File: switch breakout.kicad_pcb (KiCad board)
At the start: 2 copper layers, 2 parts

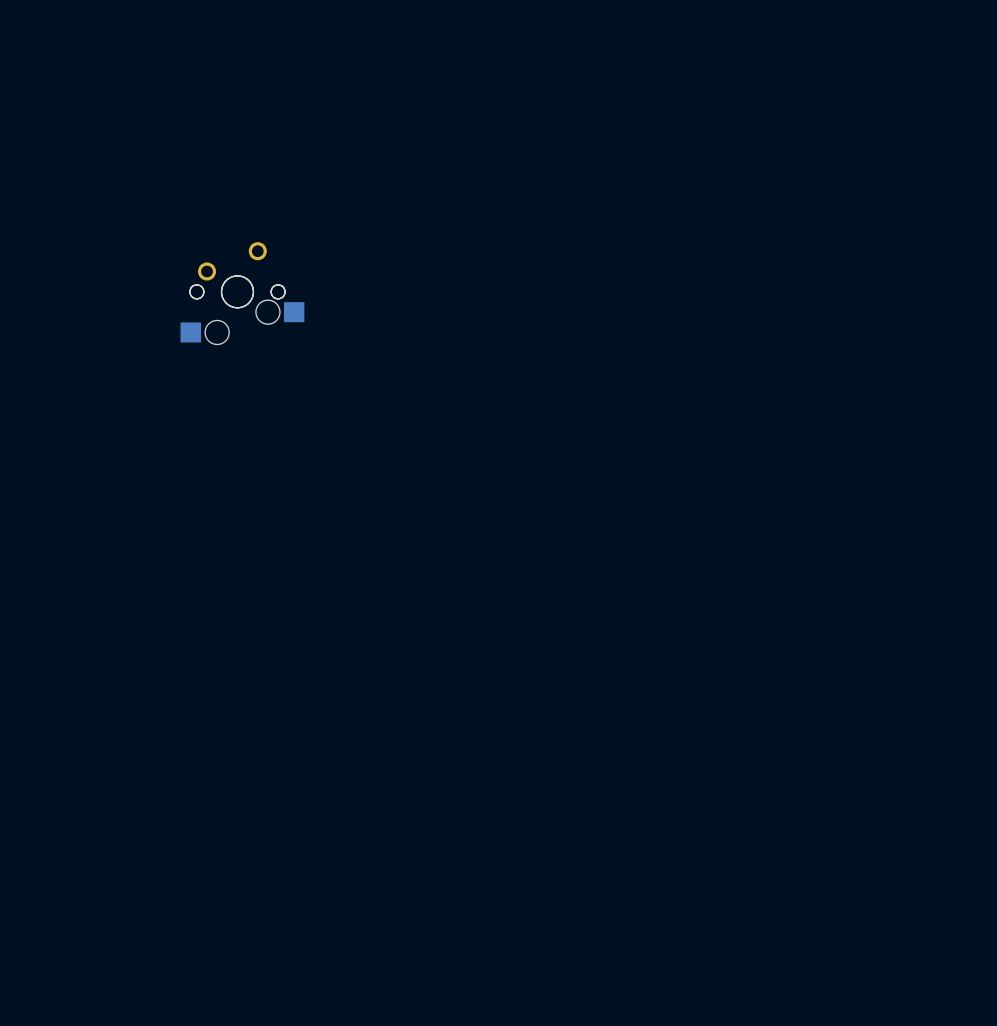
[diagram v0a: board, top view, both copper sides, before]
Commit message: update
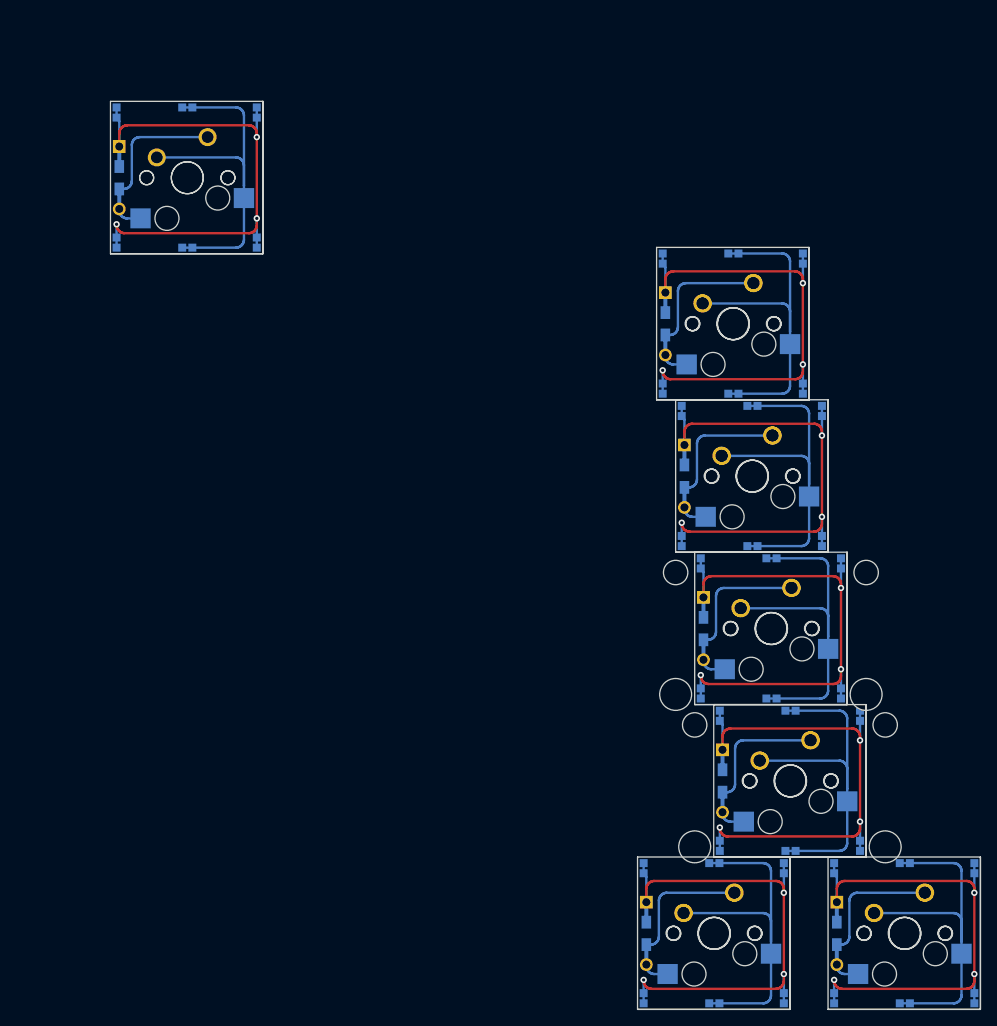
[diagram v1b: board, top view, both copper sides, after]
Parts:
- removed the MX1 at (41.3, 49.2)
- removed the REF** at (41.3, 49.2)
- added D1: 1N4148W, Keebio-Parts:Diode-dual - Copy, B.Cu at (116.2, 129.4)
- added D1: 1N4148W, Keebio-Parts:Diode-dual - Copy, B.Cu at (92.4, 129.4)
- added D1: 1N4148W, Keebio-Parts:Diode-dual - Copy, B.Cu at (101.9, 110.4)
- added D1: 1N4148W, Keebio-Parts:Diode-dual - Copy, B.Cu at (99.5, 91.3)
- added D1: 1N4148W, Keebio-Parts:Diode-dual - Copy, B.Cu at (97.1, 72.3)
- added D1: 1N4148W, Keebio-Parts:Diode-dual - Copy, B.Cu at (94.8, 53.2)
- added D1: 1N4148W, Keebio-Parts:Diode-dual - Copy, B.Cu at (26.5, 34.9)
- added MX1: MX-NoLED, MX_Only:MXOnly-1U-NoLED, F.Cu at (124.7, 129.4)
- added MX1: MX-NoLED, MX_Only:MXOnly-1U-NoLED, F.Cu at (100.9, 129.4)
- added MX1: MX-NoLED, MX_Only:MXOnly-1U-NoLED, F.Cu at (110.4, 110.4)
- added MX1: MX-NoLED, MX_Only:MXOnly-1U-NoLED, F.Cu at (108.0, 91.3)
- added MX1: MX-NoLED, MX_Only:MXOnly-1U-NoLED, F.Cu at (105.6, 72.3)
- added MX1: MX-NoLED, MX_Only:MXOnly-1U-NoLED, F.Cu at (103.3, 53.2)
- added MX1: MX-NoLED, MX_Only:MXOnly-1U-NoLED, F.Cu at (35.0, 34.9)
- added MX2: MX-NoLED, MX_Only:MXOnly-1U-Hotswap, F.Cu at (124.7, 129.4)
- added MX2: MX-NoLED, MX_Only:MXOnly-1U-Hotswap, F.Cu at (100.9, 129.4)
- added MX2: MX-NoLED, MX_Only:MXOnly-1U-Hotswap, F.Cu at (110.4, 110.4)
- added MX2: MX-NoLED, MX_Only:MXOnly-1U-Hotswap, F.Cu at (108.0, 91.3)
- added MX2: MX-NoLED, MX_Only:MXOnly-1U-Hotswap, F.Cu at (105.6, 72.3)
- added MX2: MX-NoLED, MX_Only:MXOnly-1U-Hotswap, F.Cu at (103.3, 53.2)
- added MX2: MX-NoLED, MX_Only:MXOnly-1U-Hotswap, F.Cu at (35.0, 34.9)
- added REF**: Jumper-UserFriendly, random-keyboard-parts:Jumper-UserFriendly, B.Cu at (115.9, 121.4)
- added REF**: Jumper-UserFriendly, random-keyboard-parts:Jumper-UserFriendly, B.Cu at (92.0, 121.4)
- added REF**: Jumper-UserFriendly, random-keyboard-parts:Jumper-UserFriendly, B.Cu at (109.6, 137.6)
- added REF**: Jumper-UserFriendly, random-keyboard-parts:Jumper-UserFriendly, B.Cu at (109.6, 121.4)
- added REF**: Jumper-UserFriendly, random-keyboard-parts:Jumper-UserFriendly, B.Cu at (101.6, 118.6)
- added REF**: Jumper-UserFriendly, random-keyboard-parts:Jumper-UserFriendly, B.Cu at (119.1, 118.6)
- added REF**: Jumper-UserFriendly, random-keyboard-parts:Jumper-UserFriendly, B.Cu at (110.5, 119.1)
- added REF**: Jumper-UserFriendly, random-keyboard-parts:Jumper-UserFriendly, B.Cu at (110.5, 101.6)
- added REF**: Jumper-UserFriendly, random-keyboard-parts:Jumper-UserFriendly, B.Cu at (119.1, 102.3)
- added REF**: Jumper-UserFriendly, random-keyboard-parts:Jumper-UserFriendly, B.Cu at (101.6, 102.3)
- added REF**: Jumper-UserFriendly, random-keyboard-parts:Jumper-UserFriendly, B.Cu at (99.2, 99.5)
- added REF**: Jumper-UserFriendly, random-keyboard-parts:Jumper-UserFriendly, B.Cu at (133.4, 121.4)
- added REF**: Jumper-UserFriendly, random-keyboard-parts:Jumper-UserFriendly, B.Cu at (99.2, 83.3)
- added REF**: Jumper-UserFriendly, random-keyboard-parts:Jumper-UserFriendly, B.Cu at (116.7, 99.5)
- added REF**: Jumper-UserFriendly, random-keyboard-parts:Jumper-UserFriendly, B.Cu at (116.7, 83.3)
- added REF**: Jumper-UserFriendly, random-keyboard-parts:Jumper-UserFriendly, B.Cu at (108.2, 100.0)
- added REF**: Jumper-UserFriendly, random-keyboard-parts:Jumper-UserFriendly, B.Cu at (108.2, 82.5)
- added REF**: Jumper-UserFriendly, random-keyboard-parts:Jumper-UserFriendly, B.Cu at (96.8, 80.5)
- added REF**: Jumper-UserFriendly, random-keyboard-parts:Jumper-UserFriendly, B.Cu at (96.8, 64.2)
- added REF**: Jumper-UserFriendly, random-keyboard-parts:Jumper-UserFriendly, B.Cu at (114.3, 80.5)
- added REF**: Jumper-UserFriendly, random-keyboard-parts:Jumper-UserFriendly, B.Cu at (114.3, 64.2)
- added REF**: Jumper-UserFriendly, random-keyboard-parts:Jumper-UserFriendly, B.Cu at (105.8, 63.5)
- added REF**: Jumper-UserFriendly, random-keyboard-parts:Jumper-UserFriendly, B.Cu at (133.4, 137.6)
- added REF**: Jumper-UserFriendly, random-keyboard-parts:Jumper-UserFriendly, B.Cu at (105.8, 81.0)
- added REF**: Jumper-UserFriendly, random-keyboard-parts:Jumper-UserFriendly, B.Cu at (94.4, 61.4)
- added REF**: Jumper-UserFriendly, random-keyboard-parts:Jumper-UserFriendly, B.Cu at (94.4, 45.2)
- added REF**: Jumper-UserFriendly, random-keyboard-parts:Jumper-UserFriendly, B.Cu at (112.0, 61.4)
- added REF**: Jumper-UserFriendly, random-keyboard-parts:Jumper-UserFriendly, B.Cu at (112.0, 45.2)
- added REF**: Jumper-UserFriendly, random-keyboard-parts:Jumper-UserFriendly, B.Cu at (103.4, 61.9)
- added REF**: Jumper-UserFriendly, random-keyboard-parts:Jumper-UserFriendly, B.Cu at (103.4, 44.4)
- added REF**: 2U, MX_Only:MXOnly-2U-NoLED, F.Cu at (108.0, 91.3)
- added REF**: 1.25U, MX_Only:MXOnly-1.25U-NoLED, F.Cu at (124.6, 129.4)
- added REF**: 1.25U, MX_Only:MXOnly-1.25U-NoLED, F.Cu at (100.8, 129.4)
- added REF**: Jumper-UserFriendly, random-keyboard-parts:Jumper-UserFriendly, B.Cu at (124.8, 120.6)
- added REF**: 2.25U, MX_Only:MXOnly-2.25U-NoLED, F.Cu at (110.3, 110.3)
- added REF**: 1.75U, MX_Only:MXOnly-1.75U-NoLED, F.Cu at (105.6, 72.2)
- added REF**: 1.5U, MX_Only:MXOnly-1.5U-NoLED, F.Cu at (103.2, 53.2)
- added REF**: Jumper-UserFriendly, random-keyboard-parts:Jumper-UserFriendly, B.Cu at (35.1, 26.2)
- added REF**: Jumper-UserFriendly, random-keyboard-parts:Jumper-UserFriendly, B.Cu at (35.1, 43.7)
- added REF**: Jumper-UserFriendly, random-keyboard-parts:Jumper-UserFriendly, B.Cu at (26.2, 43.2)
- added REF**: Jumper-UserFriendly, random-keyboard-parts:Jumper-UserFriendly, B.Cu at (26.2, 26.9)
- added REF**: Jumper-UserFriendly, random-keyboard-parts:Jumper-UserFriendly, B.Cu at (43.7, 26.9)
- added REF**: Jumper-UserFriendly, random-keyboard-parts:Jumper-UserFriendly, B.Cu at (43.7, 43.2)
- added REF**: Jumper-UserFriendly, random-keyboard-parts:Jumper-UserFriendly, B.Cu at (115.9, 137.6)
- added REF**: Jumper-UserFriendly, random-keyboard-parts:Jumper-UserFriendly, B.Cu at (124.8, 138.1)
- added REF**: Jumper-UserFriendly, random-keyboard-parts:Jumper-UserFriendly, B.Cu at (92.0, 137.6)
- added REF**: Jumper-UserFriendly, random-keyboard-parts:Jumper-UserFriendly, B.Cu at (101.0, 120.6)
- added REF**: Jumper-UserFriendly, random-keyboard-parts:Jumper-UserFriendly, B.Cu at (101.0, 138.1)
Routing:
- net Net-(D1-Pad1): track 0.00 -> 458.9 mm, vias 0 -> 21
- net Net-(MX1-Pad1): track 0.00 -> 322.7 mm
- net Net-(D1-Pad2): track 0.00 -> 140.5 mm
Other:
- board outline added: 108.7 x 113.5 mm
- board text added: "COL"
- board text added: "ROW"

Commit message: update
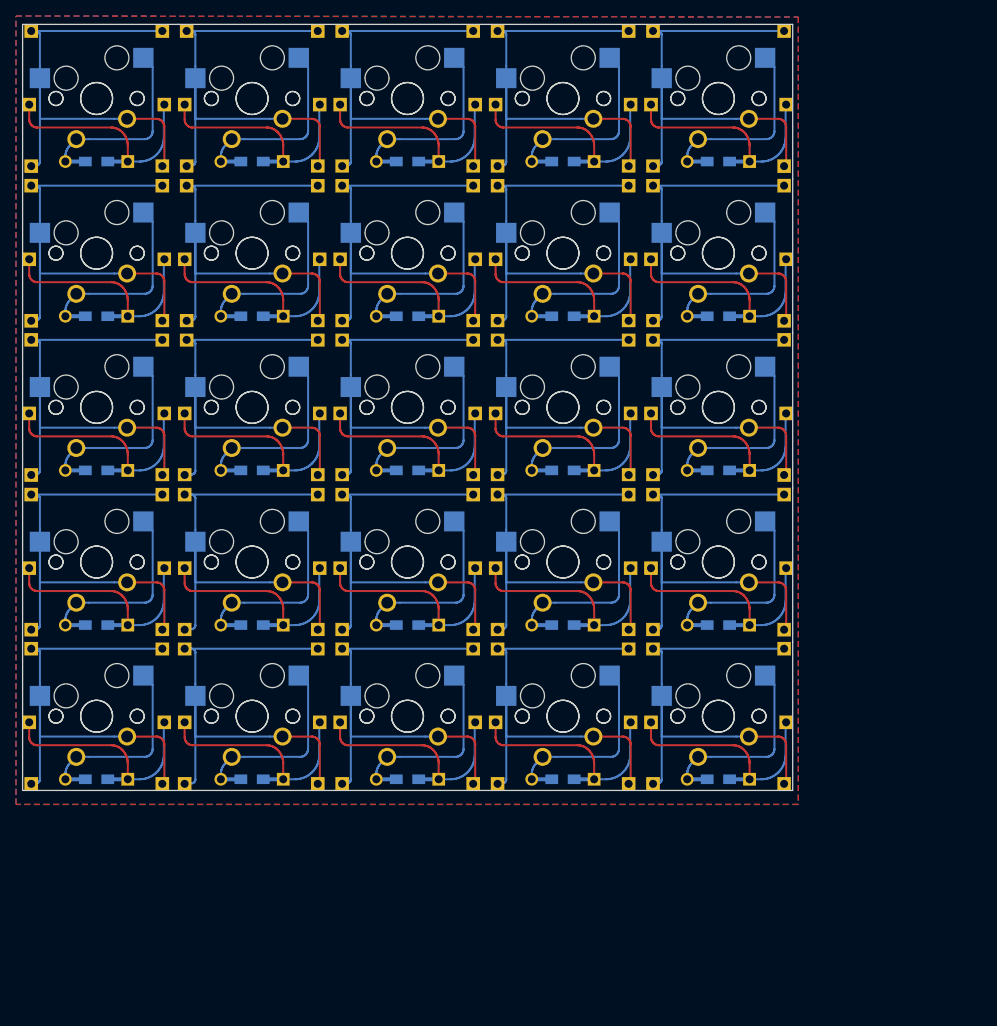
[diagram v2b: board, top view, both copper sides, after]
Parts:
- removed the D1 at (116.2, 129.4)
- removed the D1 at (92.4, 129.4)
- removed the D1 at (101.9, 110.4)
- removed the D1 at (99.5, 91.3)
- removed the D1 at (97.1, 72.3)
- removed the D1 at (94.8, 53.2)
- removed the D1 at (26.5, 34.9)
- removed the MX1 at (124.7, 129.4)
- removed the MX1 at (100.9, 129.4)
- removed the MX1 at (110.4, 110.4)
- removed the MX1 at (108.0, 91.3)
- removed the MX1 at (105.6, 72.3)
- removed the MX1 at (103.3, 53.2)
- removed the MX1 at (35.0, 34.9)
- removed the MX2 at (124.7, 129.4)
- removed the MX2 at (100.9, 129.4)
- removed the MX2 at (110.4, 110.4)
- removed the MX2 at (108.0, 91.3)
- removed the MX2 at (105.6, 72.3)
- removed the MX2 at (103.3, 53.2)
- removed the MX2 at (35.0, 34.9)
- removed the REF** at (115.9, 121.4)
- removed the REF** at (92.0, 121.4)
- removed the REF** at (109.6, 137.6)
- removed the REF** at (109.6, 121.4)
- removed the REF** at (101.6, 118.6)
- removed the REF** at (119.1, 118.6)
- removed the REF** at (110.5, 119.1)
- removed the REF** at (110.5, 101.6)
- removed the REF** at (119.1, 102.3)
- removed the REF** at (101.6, 102.3)
- removed the REF** at (99.2, 99.5)
- removed the REF** at (133.4, 121.4)
- removed the REF** at (99.2, 83.3)
- removed the REF** at (116.7, 99.5)
- removed the REF** at (116.7, 83.3)
- removed the REF** at (108.2, 100.0)
- removed the REF** at (108.2, 82.5)
- removed the REF** at (96.8, 80.5)
- removed the REF** at (96.8, 64.2)
- removed the REF** at (114.3, 80.5)
- removed the REF** at (114.3, 64.2)
- removed the REF** at (105.8, 63.5)
- removed the REF** at (133.4, 137.6)
- removed the REF** at (105.8, 81.0)
- removed the REF** at (94.4, 61.4)
- removed the REF** at (94.4, 45.2)
- removed the REF** at (112.0, 61.4)
- removed the REF** at (112.0, 45.2)
- removed the REF** at (103.4, 61.9)
- removed the REF** at (103.4, 44.4)
- removed the REF** at (108.0, 91.3)
- removed the REF** at (124.6, 129.4)
- removed the REF** at (100.8, 129.4)
- removed the REF** at (124.8, 120.6)
- removed the REF** at (110.3, 110.3)
- removed the REF** at (105.6, 72.2)
- removed the REF** at (103.2, 53.2)
- removed the REF** at (35.1, 26.2)
- removed the REF** at (35.1, 43.7)
- removed the REF** at (26.2, 43.2)
- removed the REF** at (26.2, 26.9)
- removed the REF** at (43.7, 26.9)
- removed the REF** at (43.7, 43.2)
- removed the REF** at (115.9, 137.6)
- removed the REF** at (124.8, 138.1)
- removed the REF** at (92.0, 137.6)
- removed the REF** at (101.0, 120.6)
- removed the REF** at (101.0, 138.1)
- added D1: 1N4148W, Keebio-Parts:Diode-dual - Copy, B.Cu at (62.5, 110.1)
- added D1: 1N4148W, Keebio-Parts:Diode-dual - Copy, B.Cu at (43.1, 71.5)
- added D1: 1N4148W, Keebio-Parts:Diode-dual - Copy, B.Cu at (101.4, 90.9)
- added D1: 1N4148W, Keebio-Parts:Diode-dual - Copy, B.Cu at (101.4, 71.5)
- added D1: 1N4148W, Keebio-Parts:Diode-dual - Copy, B.Cu at (82.0, 90.9)
- added D1: 1N4148W, Keebio-Parts:Diode-dual - Copy, B.Cu at (82.0, 71.5)
- added D1: 1N4148W, Keebio-Parts:Diode-dual - Copy, B.Cu at (23.7, 71.5)
- added D1: 1N4148W, Keebio-Parts:Diode-dual - Copy, B.Cu at (101.4, 52.3)
- added D1: 1N4148W, Keebio-Parts:Diode-dual - Copy, B.Cu at (101.4, 32.9)
- added D1: 1N4148W, Keebio-Parts:Diode-dual - Copy, B.Cu at (82.0, 52.3)
- added D1: 1N4148W, Keebio-Parts:Diode-dual - Copy, B.Cu at (82.0, 32.9)
- added D1: 1N4148W, Keebio-Parts:Diode-dual - Copy, B.Cu at (43.1, 110.1)
- added D1: 1N4148W, Keebio-Parts:Diode-dual - Copy, B.Cu at (62.5, 52.3)
- added D1: 1N4148W, Keebio-Parts:Diode-dual - Copy, B.Cu at (62.5, 32.9)
- added D1: 1N4148W, Keebio-Parts:Diode-dual - Copy, B.Cu at (43.1, 52.3)
- added D1: 1N4148W, Keebio-Parts:Diode-dual - Copy, B.Cu at (23.7, 52.3)
- added D1: 1N4148W, Keebio-Parts:Diode-dual - Copy, B.Cu at (43.1, 32.9)
- added D1: 1N4148W, Keebio-Parts:Diode-dual - Copy, B.Cu at (23.7, 32.9)
- added D1: 1N4148W, Keebio-Parts:Diode-dual - Copy, B.Cu at (101.4, 110.1)
- added D1: 1N4148W, Keebio-Parts:Diode-dual - Copy, B.Cu at (23.7, 110.1)
- added D1: 1N4148W, Keebio-Parts:Diode-dual - Copy, B.Cu at (82.0, 110.1)
- added D1: 1N4148W, Keebio-Parts:Diode-dual - Copy, B.Cu at (62.5, 90.9)
- added D1: 1N4148W, Keebio-Parts:Diode-dual - Copy, B.Cu at (62.5, 71.5)
- added D1: 1N4148W, Keebio-Parts:Diode-dual - Copy, B.Cu at (23.7, 90.9)
- added D1: 1N4148W, Keebio-Parts:Diode-dual - Copy, B.Cu at (43.1, 90.9)
- added MX1: MX-NoLED, MX_Only:MXOnly-1U-NoLED, F.Cu at (62.5, 102.3)
- added MX1: MX-NoLED, MX_Only:MXOnly-1U-NoLED, F.Cu at (43.1, 63.7)
- added MX1: MX-NoLED, MX_Only:MXOnly-1U-NoLED, F.Cu at (101.4, 83.0)
- added MX1: MX-NoLED, MX_Only:MXOnly-1U-NoLED, F.Cu at (101.4, 63.7)
- added MX1: MX-NoLED, MX_Only:MXOnly-1U-NoLED, F.Cu at (82.0, 83.0)
- added MX1: MX-NoLED, MX_Only:MXOnly-1U-NoLED, F.Cu at (82.0, 63.7)
- added MX1: MX-NoLED, MX_Only:MXOnly-1U-NoLED, F.Cu at (23.7, 63.7)
- added MX1: MX-NoLED, MX_Only:MXOnly-1U-NoLED, F.Cu at (101.4, 44.4)
- added MX1: MX-NoLED, MX_Only:MXOnly-1U-NoLED, F.Cu at (101.4, 25.0)
- added MX1: MX-NoLED, MX_Only:MXOnly-1U-NoLED, F.Cu at (82.0, 25.0)
- added MX1: MX-NoLED, MX_Only:MXOnly-1U-NoLED, F.Cu at (82.0, 44.4)
- added MX1: MX-NoLED, MX_Only:MXOnly-1U-NoLED, F.Cu at (101.4, 102.3)
- added MX1: MX-NoLED, MX_Only:MXOnly-1U-NoLED, F.Cu at (62.5, 25.0)
- added MX1: MX-NoLED, MX_Only:MXOnly-1U-NoLED, F.Cu at (62.5, 44.4)
- added MX1: MX-NoLED, MX_Only:MXOnly-1U-NoLED, F.Cu at (43.1, 44.4)
- added MX1: MX-NoLED, MX_Only:MXOnly-1U-NoLED, F.Cu at (23.7, 44.4)
- added MX1: MX-NoLED, MX_Only:MXOnly-1U-NoLED, F.Cu at (43.1, 25.0)
- added MX1: MX-NoLED, MX_Only:MXOnly-1U-NoLED, F.Cu at (23.7, 25.0)
- added MX1: MX-NoLED, MX_Only:MXOnly-1U-NoLED, F.Cu at (43.1, 102.3)
- added MX1: MX-NoLED, MX_Only:MXOnly-1U-NoLED, F.Cu at (82.0, 102.3)
- added MX1: MX-NoLED, MX_Only:MXOnly-1U-NoLED, F.Cu at (23.7, 102.3)
- added MX1: MX-NoLED, MX_Only:MXOnly-1U-NoLED, F.Cu at (62.5, 63.7)
- added MX1: MX-NoLED, MX_Only:MXOnly-1U-NoLED, F.Cu at (62.5, 83.0)
- added MX1: MX-NoLED, MX_Only:MXOnly-1U-NoLED, F.Cu at (43.1, 83.0)
- added MX1: MX-NoLED, MX_Only:MXOnly-1U-NoLED, F.Cu at (23.7, 83.0)
- added MX2: MX-NoLED, MX_Only:MXOnly-1U-Hotswap, F.Cu at (82.0, 25.0)
- added MX2: MX-NoLED, MX_Only:MXOnly-1U-Hotswap, F.Cu at (43.1, 83.0)
- added MX2: MX-NoLED, MX_Only:MXOnly-1U-Hotswap, F.Cu at (43.1, 63.7)
- added MX2: MX-NoLED, MX_Only:MXOnly-1U-Hotswap, F.Cu at (101.4, 63.7)
- added MX2: MX-NoLED, MX_Only:MXOnly-1U-Hotswap, F.Cu at (101.4, 83.0)
- added MX2: MX-NoLED, MX_Only:MXOnly-1U-Hotswap, F.Cu at (82.0, 83.0)
- added MX2: MX-NoLED, MX_Only:MXOnly-1U-Hotswap, F.Cu at (82.0, 63.7)
- added MX2: MX-NoLED, MX_Only:MXOnly-1U-Hotswap, F.Cu at (23.7, 63.7)
- added MX2: MX-NoLED, MX_Only:MXOnly-1U-Hotswap, F.Cu at (101.4, 44.4)
- added MX2: MX-NoLED, MX_Only:MXOnly-1U-Hotswap, F.Cu at (101.4, 25.0)
- added MX2: MX-NoLED, MX_Only:MXOnly-1U-Hotswap, F.Cu at (82.0, 44.4)
- added MX2: MX-NoLED, MX_Only:MXOnly-1U-Hotswap, F.Cu at (62.5, 102.3)
- added MX2: MX-NoLED, MX_Only:MXOnly-1U-Hotswap, F.Cu at (62.5, 25.0)
- added MX2: MX-NoLED, MX_Only:MXOnly-1U-Hotswap, F.Cu at (62.5, 44.4)
- added MX2: MX-NoLED, MX_Only:MXOnly-1U-Hotswap, F.Cu at (43.1, 44.4)
- added MX2: MX-NoLED, MX_Only:MXOnly-1U-Hotswap, F.Cu at (23.7, 44.4)
- added MX2: MX-NoLED, MX_Only:MXOnly-1U-Hotswap, F.Cu at (43.1, 25.0)
- added MX2: MX-NoLED, MX_Only:MXOnly-1U-Hotswap, F.Cu at (23.7, 25.0)
- added MX2: MX-NoLED, MX_Only:MXOnly-1U-Hotswap, F.Cu at (43.1, 102.3)
- added MX2: MX-NoLED, MX_Only:MXOnly-1U-Hotswap, F.Cu at (101.4, 102.3)
- added MX2: MX-NoLED, MX_Only:MXOnly-1U-Hotswap, F.Cu at (82.0, 102.3)
- added MX2: MX-NoLED, MX_Only:MXOnly-1U-Hotswap, F.Cu at (23.7, 102.3)
- added MX2: MX-NoLED, MX_Only:MXOnly-1U-Hotswap, F.Cu at (62.5, 63.7)
- added MX2: MX-NoLED, MX_Only:MXOnly-1U-Hotswap, F.Cu at (62.5, 83.0)
- added MX2: MX-NoLED, MX_Only:MXOnly-1U-Hotswap, F.Cu at (23.7, 83.0)
- added REF**: breakaway-mousebites, random-keyboard-parts:breakaway-mousebites, F.Cu at (33.4, 63.8)
- added REF**: breakaway-mousebites, random-keyboard-parts:breakaway-mousebites, F.Cu at (52.8, 44.5)
- added REF**: PinHeader_1x01_P2.54mm_Vertical, Connector_PinHeader_2.54mm:PinHeader_1x01_P2.54mm_Vertical, F.Cu at (35.1, 64.9)
- added REF**: PinHeader_1x01_P2.54mm_Vertical, Connector_PinHeader_2.54mm:PinHeader_1x01_P2.54mm_Vertical, F.Cu at (51.8, 72.5)
- added REF**: PinHeader_1x01_P2.54mm_Vertical, Connector_PinHeader_2.54mm:PinHeader_1x01_P2.54mm_Vertical, F.Cu at (51.8, 55.7)
- added REF**: PinHeader_1x01_P2.54mm_Vertical, Connector_PinHeader_2.54mm:PinHeader_1x01_P2.54mm_Vertical, F.Cu at (35.1, 72.5)
- added REF**: PinHeader_1x01_P2.54mm_Vertical, Connector_PinHeader_2.54mm:PinHeader_1x01_P2.54mm_Vertical, F.Cu at (52.0, 64.9)
- added REF**: PinHeader_1x01_P2.54mm_Vertical, Connector_PinHeader_2.54mm:PinHeader_1x01_P2.54mm_Vertical, F.Cu at (93.7, 91.9)
- added REF**: PinHeader_1x01_P2.54mm_Vertical, Connector_PinHeader_2.54mm:PinHeader_1x01_P2.54mm_Vertical, F.Cu at (110.0, 72.5)
- added REF**: PinHeader_1x01_P2.54mm_Vertical, Connector_PinHeader_2.54mm:PinHeader_1x01_P2.54mm_Vertical, F.Cu at (93.7, 55.7)
- added REF**: PinHeader_1x01_P2.54mm_Vertical, Connector_PinHeader_2.54mm:PinHeader_1x01_P2.54mm_Vertical, F.Cu at (93.7, 72.5)
- added REF**: PinHeader_1x01_P2.54mm_Vertical, Connector_PinHeader_2.54mm:PinHeader_1x01_P2.54mm_Vertical, F.Cu at (93.7, 75.0)
- added REF**: breakaway-mousebites, random-keyboard-parts:breakaway-mousebites, F.Cu at (72.3, 63.8)
- added REF**: PinHeader_1x01_P2.54mm_Vertical, Connector_PinHeader_2.54mm:PinHeader_1x01_P2.54mm_Vertical, F.Cu at (110.0, 55.7)
- added REF**: PinHeader_1x01_P2.54mm_Vertical, Connector_PinHeader_2.54mm:PinHeader_1x01_P2.54mm_Vertical, F.Cu at (93.4, 64.9)
- added REF**: PinHeader_1x01_P2.54mm_Vertical, Connector_PinHeader_2.54mm:PinHeader_1x01_P2.54mm_Vertical, F.Cu at (110.3, 64.9)
- added REF**: PinHeader_1x01_P2.54mm_Vertical, Connector_PinHeader_2.54mm:PinHeader_1x01_P2.54mm_Vertical, F.Cu at (110.3, 84.2)
- added REF**: PinHeader_1x01_P2.54mm_Vertical, Connector_PinHeader_2.54mm:PinHeader_1x01_P2.54mm_Vertical, F.Cu at (110.0, 75.0)
- added REF**: PinHeader_1x01_P2.54mm_Vertical, Connector_PinHeader_2.54mm:PinHeader_1x01_P2.54mm_Vertical, F.Cu at (93.4, 84.2)
- added REF**: PinHeader_1x01_P2.54mm_Vertical, Connector_PinHeader_2.54mm:PinHeader_1x01_P2.54mm_Vertical, F.Cu at (74.2, 55.7)
- added REF**: PinHeader_1x01_P2.54mm_Vertical, Connector_PinHeader_2.54mm:PinHeader_1x01_P2.54mm_Vertical, F.Cu at (90.6, 72.5)
- added REF**: PinHeader_1x01_P2.54mm_Vertical, Connector_PinHeader_2.54mm:PinHeader_1x01_P2.54mm_Vertical, F.Cu at (74.2, 91.9)
- added REF**: PinHeader_1x01_P2.54mm_Vertical, Connector_PinHeader_2.54mm:PinHeader_1x01_P2.54mm_Vertical, F.Cu at (74.2, 72.5)
- added REF**: breakaway-mousebites, random-keyboard-parts:breakaway-mousebites, F.Cu at (52.8, 63.8)
- added REF**: PinHeader_1x01_P2.54mm_Vertical, Connector_PinHeader_2.54mm:PinHeader_1x01_P2.54mm_Vertical, F.Cu at (74.2, 75.0)
- added REF**: PinHeader_1x01_P2.54mm_Vertical, Connector_PinHeader_2.54mm:PinHeader_1x01_P2.54mm_Vertical, F.Cu at (90.6, 55.7)
- added REF**: PinHeader_1x01_P2.54mm_Vertical, Connector_PinHeader_2.54mm:PinHeader_1x01_P2.54mm_Vertical, F.Cu at (110.0, 91.9)
- added REF**: PinHeader_1x01_P2.54mm_Vertical, Connector_PinHeader_2.54mm:PinHeader_1x01_P2.54mm_Vertical, F.Cu at (74.0, 64.9)
- added REF**: PinHeader_1x01_P2.54mm_Vertical, Connector_PinHeader_2.54mm:PinHeader_1x01_P2.54mm_Vertical, F.Cu at (90.9, 64.9)
- added REF**: PinHeader_1x01_P2.54mm_Vertical, Connector_PinHeader_2.54mm:PinHeader_1x01_P2.54mm_Vertical, F.Cu at (90.9, 84.2)
- added REF**: PinHeader_1x01_P2.54mm_Vertical, Connector_PinHeader_2.54mm:PinHeader_1x01_P2.54mm_Vertical, F.Cu at (90.6, 75.0)
- added REF**: PinHeader_1x01_P2.54mm_Vertical, Connector_PinHeader_2.54mm:PinHeader_1x01_P2.54mm_Vertical, F.Cu at (74.0, 84.2)
- added REF**: PinHeader_1x01_P2.54mm_Vertical, Connector_PinHeader_2.54mm:PinHeader_1x01_P2.54mm_Vertical, F.Cu at (90.6, 91.9)
- added REF**: PinHeader_1x01_P2.54mm_Vertical, Connector_PinHeader_2.54mm:PinHeader_1x01_P2.54mm_Vertical, F.Cu at (54.5, 84.2)
- added REF**: breakaway-mousebites, random-keyboard-parts:breakaway-mousebites, F.Cu at (91.7, 63.8)
- added REF**: PinHeader_1x01_P2.54mm_Vertical, Connector_PinHeader_2.54mm:PinHeader_1x01_P2.54mm_Vertical, F.Cu at (71.2, 75.0)
- added REF**: PinHeader_1x01_P2.54mm_Vertical, Connector_PinHeader_2.54mm:PinHeader_1x01_P2.54mm_Vertical, F.Cu at (15.9, 55.7)
- added REF**: PinHeader_1x01_P2.54mm_Vertical, Connector_PinHeader_2.54mm:PinHeader_1x01_P2.54mm_Vertical, F.Cu at (15.7, 64.9)
- added REF**: PinHeader_1x01_P2.54mm_Vertical, Connector_PinHeader_2.54mm:PinHeader_1x01_P2.54mm_Vertical, F.Cu at (15.9, 72.5)
- added REF**: PinHeader_1x01_P2.54mm_Vertical, Connector_PinHeader_2.54mm:PinHeader_1x01_P2.54mm_Vertical, F.Cu at (32.3, 72.5)
- added REF**: PinHeader_1x01_P2.54mm_Vertical, Connector_PinHeader_2.54mm:PinHeader_1x01_P2.54mm_Vertical, F.Cu at (32.3, 55.7)
- added REF**: PinHeader_1x01_P2.54mm_Vertical, Connector_PinHeader_2.54mm:PinHeader_1x01_P2.54mm_Vertical, F.Cu at (32.6, 64.9)
- added REF**: PinHeader_1x01_P2.54mm_Vertical, Connector_PinHeader_2.54mm:PinHeader_1x01_P2.54mm_Vertical, F.Cu at (93.7, 17.0)
- added REF**: PinHeader_1x01_P2.54mm_Vertical, Connector_PinHeader_2.54mm:PinHeader_1x01_P2.54mm_Vertical, F.Cu at (110.0, 33.9)
- added REF**: PinHeader_1x01_P2.54mm_Vertical, Connector_PinHeader_2.54mm:PinHeader_1x01_P2.54mm_Vertical, F.Cu at (93.7, 53.3)
- added REF**: breakaway-mousebites, random-keyboard-parts:breakaway-mousebites, F.Cu at (72.3, 83.2)
- added REF**: PinHeader_1x01_P2.54mm_Vertical, Connector_PinHeader_2.54mm:PinHeader_1x01_P2.54mm_Vertical, F.Cu at (93.7, 33.9)
- added REF**: PinHeader_1x01_P2.54mm_Vertical, Connector_PinHeader_2.54mm:PinHeader_1x01_P2.54mm_Vertical, F.Cu at (93.7, 36.4)
- added REF**: PinHeader_1x01_P2.54mm_Vertical, Connector_PinHeader_2.54mm:PinHeader_1x01_P2.54mm_Vertical, F.Cu at (110.0, 17.0)
- added REF**: PinHeader_1x01_P2.54mm_Vertical, Connector_PinHeader_2.54mm:PinHeader_1x01_P2.54mm_Vertical, F.Cu at (93.4, 26.2)
- added REF**: PinHeader_1x01_P2.54mm_Vertical, Connector_PinHeader_2.54mm:PinHeader_1x01_P2.54mm_Vertical, F.Cu at (110.3, 26.2)
- added REF**: PinHeader_1x01_P2.54mm_Vertical, Connector_PinHeader_2.54mm:PinHeader_1x01_P2.54mm_Vertical, F.Cu at (110.3, 45.6)
- added REF**: PinHeader_1x01_P2.54mm_Vertical, Connector_PinHeader_2.54mm:PinHeader_1x01_P2.54mm_Vertical, F.Cu at (110.0, 36.4)
- added REF**: PinHeader_1x01_P2.54mm_Vertical, Connector_PinHeader_2.54mm:PinHeader_1x01_P2.54mm_Vertical, F.Cu at (93.4, 45.6)
- added REF**: PinHeader_1x01_P2.54mm_Vertical, Connector_PinHeader_2.54mm:PinHeader_1x01_P2.54mm_Vertical, F.Cu at (110.0, 53.3)
- added REF**: PinHeader_1x01_P2.54mm_Vertical, Connector_PinHeader_2.54mm:PinHeader_1x01_P2.54mm_Vertical, F.Cu at (90.6, 17.0)
- added REF**: breakaway-mousebites, random-keyboard-parts:breakaway-mousebites, F.Cu at (33.4, 83.2)
- added REF**: PinHeader_1x01_P2.54mm_Vertical, Connector_PinHeader_2.54mm:PinHeader_1x01_P2.54mm_Vertical, F.Cu at (90.9, 45.6)
- added REF**: PinHeader_1x01_P2.54mm_Vertical, Connector_PinHeader_2.54mm:PinHeader_1x01_P2.54mm_Vertical, F.Cu at (90.9, 26.2)
- added REF**: PinHeader_1x01_P2.54mm_Vertical, Connector_PinHeader_2.54mm:PinHeader_1x01_P2.54mm_Vertical, F.Cu at (90.6, 33.9)
- added REF**: PinHeader_1x01_P2.54mm_Vertical, Connector_PinHeader_2.54mm:PinHeader_1x01_P2.54mm_Vertical, F.Cu at (74.2, 17.0)
- added REF**: PinHeader_1x01_P2.54mm_Vertical, Connector_PinHeader_2.54mm:PinHeader_1x01_P2.54mm_Vertical, F.Cu at (74.2, 36.4)
- added REF**: PinHeader_1x01_P2.54mm_Vertical, Connector_PinHeader_2.54mm:PinHeader_1x01_P2.54mm_Vertical, F.Cu at (74.2, 53.3)
- added REF**: PinHeader_1x01_P2.54mm_Vertical, Connector_PinHeader_2.54mm:PinHeader_1x01_P2.54mm_Vertical, F.Cu at (74.2, 33.9)
- added REF**: PinHeader_1x01_P2.54mm_Vertical, Connector_PinHeader_2.54mm:PinHeader_1x01_P2.54mm_Vertical, F.Cu at (74.0, 26.2)
- added REF**: PinHeader_1x01_P2.54mm_Vertical, Connector_PinHeader_2.54mm:PinHeader_1x01_P2.54mm_Vertical, F.Cu at (90.6, 53.3)
- added REF**: PinHeader_1x01_P2.54mm_Vertical, Connector_PinHeader_2.54mm:PinHeader_1x01_P2.54mm_Vertical, F.Cu at (74.0, 45.6)
- added REF**: breakaway-mousebites, random-keyboard-parts:breakaway-mousebites, F.Cu at (52.8, 83.2)
- added REF**: PinHeader_1x01_P2.54mm_Vertical, Connector_PinHeader_2.54mm:PinHeader_1x01_P2.54mm_Vertical, F.Cu at (90.6, 36.4)
- added REF**: PinHeader_1x01_P2.54mm_Vertical, Connector_PinHeader_2.54mm:PinHeader_1x01_P2.54mm_Vertical, F.Cu at (54.5, 45.6)
- added REF**: PinHeader_1x01_P2.54mm_Vertical, Connector_PinHeader_2.54mm:PinHeader_1x01_P2.54mm_Vertical, F.Cu at (71.2, 36.4)
- added REF**: PinHeader_1x01_P2.54mm_Vertical, Connector_PinHeader_2.54mm:PinHeader_1x01_P2.54mm_Vertical, F.Cu at (71.2, 17.0)
- added REF**: PinHeader_1x01_P2.54mm_Vertical, Connector_PinHeader_2.54mm:PinHeader_1x01_P2.54mm_Vertical, F.Cu at (71.4, 26.2)
- added REF**: PinHeader_1x01_P2.54mm_Vertical, Connector_PinHeader_2.54mm:PinHeader_1x01_P2.54mm_Vertical, F.Cu at (71.2, 33.9)
- added REF**: PinHeader_1x01_P2.54mm_Vertical, Connector_PinHeader_2.54mm:PinHeader_1x01_P2.54mm_Vertical, F.Cu at (71.4, 45.6)
- added REF**: PinHeader_1x01_P2.54mm_Vertical, Connector_PinHeader_2.54mm:PinHeader_1x01_P2.54mm_Vertical, F.Cu at (54.8, 17.0)
- added REF**: PinHeader_1x01_P2.54mm_Vertical, Connector_PinHeader_2.54mm:PinHeader_1x01_P2.54mm_Vertical, F.Cu at (54.8, 33.9)
- added REF**: PinHeader_1x01_P2.54mm_Vertical, Connector_PinHeader_2.54mm:PinHeader_1x01_P2.54mm_Vertical, F.Cu at (54.5, 26.2)
- added REF**: breakaway-mousebites, random-keyboard-parts:breakaway-mousebites, F.Cu at (91.7, 83.2)
- added REF**: PinHeader_1x01_P2.54mm_Vertical, Connector_PinHeader_2.54mm:PinHeader_1x01_P2.54mm_Vertical, F.Cu at (54.8, 36.4)
- added REF**: PinHeader_1x01_P2.54mm_Vertical, Connector_PinHeader_2.54mm:PinHeader_1x01_P2.54mm_Vertical, F.Cu at (71.2, 53.3)
- added REF**: PinHeader_1x01_P2.54mm_Vertical, Connector_PinHeader_2.54mm:PinHeader_1x01_P2.54mm_Vertical, F.Cu at (54.8, 53.3)
- added REF**: PinHeader_1x01_P2.54mm_Vertical, Connector_PinHeader_2.54mm:PinHeader_1x01_P2.54mm_Vertical, F.Cu at (35.4, 36.4)
- added REF**: PinHeader_1x01_P2.54mm_Vertical, Connector_PinHeader_2.54mm:PinHeader_1x01_P2.54mm_Vertical, F.Cu at (35.1, 45.6)
- added REF**: PinHeader_1x01_P2.54mm_Vertical, Connector_PinHeader_2.54mm:PinHeader_1x01_P2.54mm_Vertical, F.Cu at (51.8, 53.3)
- added REF**: PinHeader_1x01_P2.54mm_Vertical, Connector_PinHeader_2.54mm:PinHeader_1x01_P2.54mm_Vertical, F.Cu at (51.8, 36.4)
- added REF**: PinHeader_1x01_P2.54mm_Vertical, Connector_PinHeader_2.54mm:PinHeader_1x01_P2.54mm_Vertical, F.Cu at (35.4, 53.3)
- added REF**: PinHeader_1x01_P2.54mm_Vertical, Connector_PinHeader_2.54mm:PinHeader_1x01_P2.54mm_Vertical, F.Cu at (52.0, 45.6)
- added REF**: PinHeader_1x01_P2.54mm_Vertical, Connector_PinHeader_2.54mm:PinHeader_1x01_P2.54mm_Vertical, F.Cu at (15.9, 36.4)
- added REF**: breakaway-mousebites, random-keyboard-parts:breakaway-mousebites, F.Cu at (33.4, 102.4)
- added REF**: PinHeader_1x01_P2.54mm_Vertical, Connector_PinHeader_2.54mm:PinHeader_1x01_P2.54mm_Vertical, F.Cu at (15.7, 45.6)
- added REF**: PinHeader_1x01_P2.54mm_Vertical, Connector_PinHeader_2.54mm:PinHeader_1x01_P2.54mm_Vertical, F.Cu at (15.9, 53.3)
- added REF**: PinHeader_1x01_P2.54mm_Vertical, Connector_PinHeader_2.54mm:PinHeader_1x01_P2.54mm_Vertical, F.Cu at (32.3, 53.3)
- added REF**: PinHeader_1x01_P2.54mm_Vertical, Connector_PinHeader_2.54mm:PinHeader_1x01_P2.54mm_Vertical, F.Cu at (32.3, 36.4)
- added REF**: PinHeader_1x01_P2.54mm_Vertical, Connector_PinHeader_2.54mm:PinHeader_1x01_P2.54mm_Vertical, F.Cu at (32.6, 45.6)
- added REF**: PinHeader_1x01_P2.54mm_Vertical, Connector_PinHeader_2.54mm:PinHeader_1x01_P2.54mm_Vertical, F.Cu at (35.4, 17.0)
- added REF**: PinHeader_1x01_P2.54mm_Vertical, Connector_PinHeader_2.54mm:PinHeader_1x01_P2.54mm_Vertical, F.Cu at (35.1, 26.2)
- added REF**: PinHeader_1x01_P2.54mm_Vertical, Connector_PinHeader_2.54mm:PinHeader_1x01_P2.54mm_Vertical, F.Cu at (35.4, 33.9)
- added REF**: PinHeader_1x01_P2.54mm_Vertical, Connector_PinHeader_2.54mm:PinHeader_1x01_P2.54mm_Vertical, F.Cu at (51.8, 33.9)
- added REF**: PinHeader_1x01_P2.54mm_Vertical, Connector_PinHeader_2.54mm:PinHeader_1x01_P2.54mm_Vertical, F.Cu at (51.8, 17.0)
- added REF**: breakaway-mousebites, random-keyboard-parts:breakaway-mousebites, F.Cu at (52.8, 102.4)
- added REF**: PinHeader_1x01_P2.54mm_Vertical, Connector_PinHeader_2.54mm:PinHeader_1x01_P2.54mm_Vertical, F.Cu at (32.6, 26.2)
- added REF**: PinHeader_1x01_P2.54mm_Vertical, Connector_PinHeader_2.54mm:PinHeader_1x01_P2.54mm_Vertical, F.Cu at (32.3, 17.0)
- added REF**: PinHeader_1x01_P2.54mm_Vertical, Connector_PinHeader_2.54mm:PinHeader_1x01_P2.54mm_Vertical, F.Cu at (32.3, 33.9)
- added REF**: PinHeader_1x01_P2.54mm_Vertical, Connector_PinHeader_2.54mm:PinHeader_1x01_P2.54mm_Vertical, F.Cu at (15.9, 33.9)
- added REF**: PinHeader_1x01_P2.54mm_Vertical, Connector_PinHeader_2.54mm:PinHeader_1x01_P2.54mm_Vertical, F.Cu at (15.7, 26.2)
- added REF**: PinHeader_1x01_P2.54mm_Vertical, Connector_PinHeader_2.54mm:PinHeader_1x01_P2.54mm_Vertical, F.Cu at (15.9, 17.0)
- added REF**: PinHeader_1x01_P2.54mm_Vertical, Connector_PinHeader_2.54mm:PinHeader_1x01_P2.54mm_Vertical, F.Cu at (52.0, 26.2)
- added REF**: breakaway-mousebites, random-keyboard-parts:breakaway-mousebites, F.Cu at (72.3, 102.4)
- added REF**: breakaway-mousebites, random-keyboard-parts:breakaway-mousebites, F.Cu at (91.7, 102.4)
- added REF**: breakaway-mousebites, random-keyboard-parts:breakaway-mousebites, F.Cu at (33.4, 92.6)
- added REF**: breakaway-mousebites, random-keyboard-parts:breakaway-mousebites, F.Cu at (52.8, 92.6)
- added REF**: breakaway-mousebites, random-keyboard-parts:breakaway-mousebites, F.Cu at (91.7, 92.6)
- added REF**: breakaway-mousebites, random-keyboard-parts:breakaway-mousebites, F.Cu at (72.3, 92.6)
- added REF**: breakaway-mousebites, random-keyboard-parts:breakaway-mousebites, F.Cu at (33.4, 73.3)
- added REF**: breakaway-mousebites, random-keyboard-parts:breakaway-mousebites, F.Cu at (52.8, 73.3)
- added REF**: breakaway-mousebites, random-keyboard-parts:breakaway-mousebites, F.Cu at (72.3, 73.3)
- added REF**: breakaway-mousebites, random-keyboard-parts:breakaway-mousebites, F.Cu at (91.7, 73.3)
- added REF**: breakaway-mousebites, random-keyboard-parts:breakaway-mousebites, F.Cu at (72.3, 25.2)
- added REF**: breakaway-mousebites, random-keyboard-parts:breakaway-mousebites, F.Cu at (33.4, 54.0)
- added REF**: breakaway-mousebites, random-keyboard-parts:breakaway-mousebites, F.Cu at (52.8, 54.0)
- added REF**: breakaway-mousebites, random-keyboard-parts:breakaway-mousebites, F.Cu at (72.3, 54.0)
- added REF**: breakaway-mousebites, random-keyboard-parts:breakaway-mousebites, F.Cu at (91.7, 54.0)
- added REF**: breakaway-mousebites, random-keyboard-parts:breakaway-mousebites, F.Cu at (33.4, 34.7)
- added REF**: breakaway-mousebites, random-keyboard-parts:breakaway-mousebites, F.Cu at (52.8, 34.7)
- added REF**: breakaway-mousebites, random-keyboard-parts:breakaway-mousebites, F.Cu at (72.3, 34.7)
- added REF**: breakaway-mousebites, random-keyboard-parts:breakaway-mousebites, F.Cu at (91.7, 34.7)
- added REF**: breakaway-mousebites, random-keyboard-parts:breakaway-mousebites, F.Cu at (19.8, 92.6)
- added REF**: breakaway-mousebites, random-keyboard-parts:breakaway-mousebites, F.Cu at (105.3, 92.6)
- added REF**: breakaway-mousebites, random-keyboard-parts:breakaway-mousebites, F.Cu at (91.7, 25.2)
- added REF**: breakaway-mousebites, random-keyboard-parts:breakaway-mousebites, F.Cu at (19.8, 34.7)
- added REF**: breakaway-mousebites, random-keyboard-parts:breakaway-mousebites, F.Cu at (66.4, 34.7)
- added REF**: breakaway-mousebites, random-keyboard-parts:breakaway-mousebites, F.Cu at (105.3, 34.7)
- added REF**: breakaway-mousebites, random-keyboard-parts:breakaway-mousebites, F.Cu at (19.8, 54.0)
- added REF**: breakaway-mousebites, random-keyboard-parts:breakaway-mousebites, F.Cu at (105.3, 54.0)
- added REF**: breakaway-mousebites, random-keyboard-parts:breakaway-mousebites, F.Cu at (19.8, 73.3)
- added REF**: breakaway-mousebites, random-keyboard-parts:breakaway-mousebites, F.Cu at (105.3, 73.3)
- added REF**: PinHeader_1x01_P2.54mm_Vertical, Connector_PinHeader_2.54mm:PinHeader_1x01_P2.54mm_Vertical, F.Cu at (71.2, 94.3)
- added REF**: PinHeader_1x01_P2.54mm_Vertical, Connector_PinHeader_2.54mm:PinHeader_1x01_P2.54mm_Vertical, F.Cu at (71.4, 103.5)
- added REF**: PinHeader_1x01_P2.54mm_Vertical, Connector_PinHeader_2.54mm:PinHeader_1x01_P2.54mm_Vertical, F.Cu at (71.2, 111.2)
- added REF**: breakaway-mousebites, random-keyboard-parts:breakaway-mousebites, F.Cu at (33.4, 25.2)
- added REF**: PinHeader_1x01_P2.54mm_Vertical, Connector_PinHeader_2.54mm:PinHeader_1x01_P2.54mm_Vertical, F.Cu at (54.8, 94.3)
- added REF**: PinHeader_1x01_P2.54mm_Vertical, Connector_PinHeader_2.54mm:PinHeader_1x01_P2.54mm_Vertical, F.Cu at (54.8, 111.2)
- added REF**: PinHeader_1x01_P2.54mm_Vertical, Connector_PinHeader_2.54mm:PinHeader_1x01_P2.54mm_Vertical, F.Cu at (54.5, 103.5)
- added REF**: PinHeader_1x01_P2.54mm_Vertical, Connector_PinHeader_2.54mm:PinHeader_1x01_P2.54mm_Vertical, F.Cu at (110.0, 111.2)
- added REF**: PinHeader_1x01_P2.54mm_Vertical, Connector_PinHeader_2.54mm:PinHeader_1x01_P2.54mm_Vertical, F.Cu at (93.7, 94.3)
- added REF**: PinHeader_1x01_P2.54mm_Vertical, Connector_PinHeader_2.54mm:PinHeader_1x01_P2.54mm_Vertical, F.Cu at (51.8, 111.2)
- added REF**: PinHeader_1x01_P2.54mm_Vertical, Connector_PinHeader_2.54mm:PinHeader_1x01_P2.54mm_Vertical, F.Cu at (35.1, 103.5)
- added REF**: PinHeader_1x01_P2.54mm_Vertical, Connector_PinHeader_2.54mm:PinHeader_1x01_P2.54mm_Vertical, F.Cu at (52.0, 103.5)
- added REF**: PinHeader_1x01_P2.54mm_Vertical, Connector_PinHeader_2.54mm:PinHeader_1x01_P2.54mm_Vertical, F.Cu at (35.1, 111.2)
- added REF**: PinHeader_1x01_P2.54mm_Vertical, Connector_PinHeader_2.54mm:PinHeader_1x01_P2.54mm_Vertical, F.Cu at (35.1, 94.3)
- added REF**: breakaway-mousebites, random-keyboard-parts:breakaway-mousebites, F.Cu at (52.8, 25.2)
- added REF**: PinHeader_1x01_P2.54mm_Vertical, Connector_PinHeader_2.54mm:PinHeader_1x01_P2.54mm_Vertical, F.Cu at (51.8, 94.3)
- added REF**: PinHeader_1x01_P2.54mm_Vertical, Connector_PinHeader_2.54mm:PinHeader_1x01_P2.54mm_Vertical, F.Cu at (93.7, 111.2)
- added REF**: PinHeader_1x01_P2.54mm_Vertical, Connector_PinHeader_2.54mm:PinHeader_1x01_P2.54mm_Vertical, F.Cu at (93.4, 103.5)
- added REF**: PinHeader_1x01_P2.54mm_Vertical, Connector_PinHeader_2.54mm:PinHeader_1x01_P2.54mm_Vertical, F.Cu at (110.0, 94.3)
- added REF**: PinHeader_1x01_P2.54mm_Vertical, Connector_PinHeader_2.54mm:PinHeader_1x01_P2.54mm_Vertical, F.Cu at (110.3, 103.5)
- added REF**: PinHeader_1x01_P2.54mm_Vertical, Connector_PinHeader_2.54mm:PinHeader_1x01_P2.54mm_Vertical, F.Cu at (90.6, 111.2)
- added REF**: PinHeader_1x01_P2.54mm_Vertical, Connector_PinHeader_2.54mm:PinHeader_1x01_P2.54mm_Vertical, F.Cu at (74.2, 111.2)
- added REF**: PinHeader_1x01_P2.54mm_Vertical, Connector_PinHeader_2.54mm:PinHeader_1x01_P2.54mm_Vertical, F.Cu at (15.7, 103.5)
- added REF**: PinHeader_1x01_P2.54mm_Vertical, Connector_PinHeader_2.54mm:PinHeader_1x01_P2.54mm_Vertical, F.Cu at (32.3, 111.2)
- added REF**: PinHeader_1x01_P2.54mm_Vertical, Connector_PinHeader_2.54mm:PinHeader_1x01_P2.54mm_Vertical, F.Cu at (74.2, 94.3)
- added REF**: breakaway-mousebites, random-keyboard-parts:breakaway-mousebites, F.Cu at (91.7, 44.5)
- added REF**: PinHeader_1x01_P2.54mm_Vertical, Connector_PinHeader_2.54mm:PinHeader_1x01_P2.54mm_Vertical, F.Cu at (74.0, 103.5)
- added REF**: PinHeader_1x01_P2.54mm_Vertical, Connector_PinHeader_2.54mm:PinHeader_1x01_P2.54mm_Vertical, F.Cu at (15.9, 94.3)
- added REF**: PinHeader_1x01_P2.54mm_Vertical, Connector_PinHeader_2.54mm:PinHeader_1x01_P2.54mm_Vertical, F.Cu at (90.6, 94.3)
- added REF**: PinHeader_1x01_P2.54mm_Vertical, Connector_PinHeader_2.54mm:PinHeader_1x01_P2.54mm_Vertical, F.Cu at (15.9, 111.2)
- added REF**: PinHeader_1x01_P2.54mm_Vertical, Connector_PinHeader_2.54mm:PinHeader_1x01_P2.54mm_Vertical, F.Cu at (90.9, 103.5)
- added REF**: PinHeader_1x01_P2.54mm_Vertical, Connector_PinHeader_2.54mm:PinHeader_1x01_P2.54mm_Vertical, F.Cu at (32.3, 94.3)
- added REF**: PinHeader_1x01_P2.54mm_Vertical, Connector_PinHeader_2.54mm:PinHeader_1x01_P2.54mm_Vertical, F.Cu at (32.6, 103.5)
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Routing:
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- added copper zone on B.Cu, net (none)
- added copper zone on F.Cu, net (none)
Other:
- board size 108.7 x 113.5 mm -> 96.3 x 95.8 mm
- board text added: "col"
- board text added: "row"
- board text removed: "COL"
- board text removed: "ROW"
